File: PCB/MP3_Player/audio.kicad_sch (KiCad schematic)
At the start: 23 parts, among them J7 AudioPlugTRRS, J8 AudioPlugTRRS, U6 PCM5102AQPWRQ1

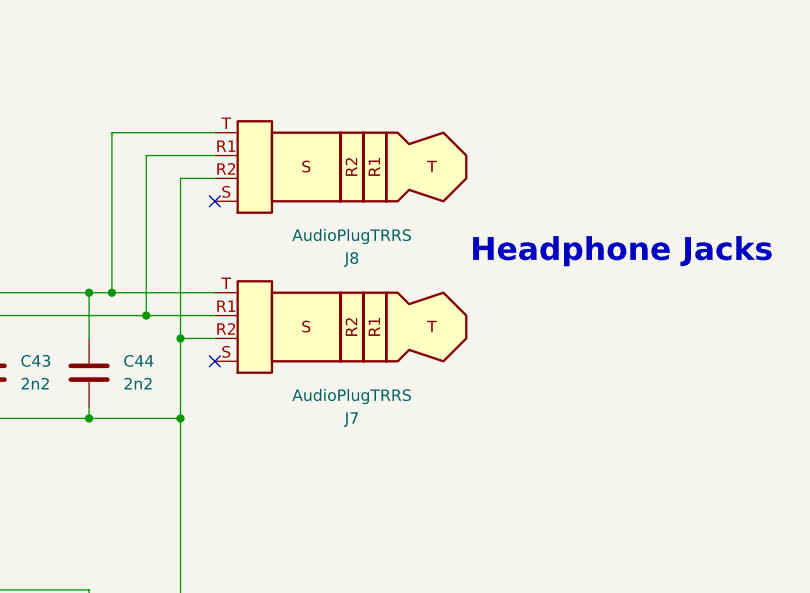
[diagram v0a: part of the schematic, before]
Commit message: PCB Routing
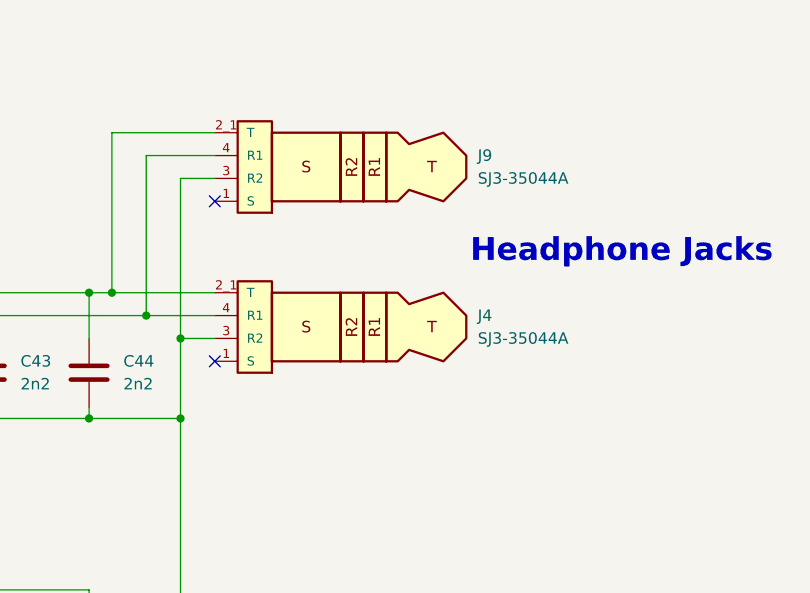
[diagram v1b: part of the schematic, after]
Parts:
- removed J7, J8: AudioPlugTRRS, SJ3-35044A:SAMESKY_SJ3-35044A, symbol Connector_Audio:AudioPlug4
- added J4, J9: SJ3-35044A, SJ3-35044A:SAMESKY_SJ3-35044A, symbol SJ3-35044A:SJ3-35044A
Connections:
- net GND: now also J4.3 (R2), J9.3 (R2)
- net LOUT: now also J4.2_1 (T), J4.2_2, J9.2_1 (T), J9.2_2
- net ROUT: now also J4.4 (R1), J9.4 (R1)

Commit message: PCB Routing
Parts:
- J4, J9: Mfr. Part # (none) -> SJ3-35044A; Store URL - Digikey (none) -> https://www.digikey.pt/pt/products/detail/same-sky-formerly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
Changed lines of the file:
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@@
 			)
 		)
-		(property "Datasheet" ""
+		(property "Datasheet" "https://www.sameskydevices.com/product/resource/sj3-35044a.pdf"
 			(at 229.87 71.12 0)
 			(hide yes)
@@
 				)
 				(justify bottom)
+			)
+		)
+		(property "Mfr. Part #" "SJ3-35044A"
+			(at 229.87 71.12 0)
+			(hide yes)
+			(show_name no)
+			(do_not_autoplace no)
+			(effects
+				(font
+					(size 1.27 1.27)
+				)
+			)
+		)
+		(property "Store URL - Digikey" "https://www.digikey.pt/pt/products/detail/same-sky-formerly-cui-devices/SJ3-35044A/24627965?s=N4IgTCBcDaIMoCkDMBaJBWADAFmwQRAF0BfIA"
+			(at 229.87 71.12 0)
+			(hide yes)
+			(show_name no)
+			(do_not_autoplace no)
+			(effects
+				(font
+					(size 1.27 1.27)
+				)
 			)
 		)
@@
 			)
 		)
-		(property "Datasheet" ""
+		(property "Datasheet" "https://www.sameskydevices.com/product/resource/sj3-35044a.pdf"
 			(at 229.87 53.34 0)
 			(hide yes)
@@
 			)
 		)
+		(property "Mfr. Part #" "SJ3-35044A"
+			(at 229.87 53.34 0)
+			(hide yes)
+			(show_name no)
+			(do_not_autoplace no)
+			(effects
+				(font
+					(size 1.27 1.27)
+				)
+			)
+		)
+		(property "Store URL - Digikey" "https://www.digikey.pt/pt/products/detail/same-sky-formerly-cui-devices/SJ3-35044A/24627965?s=N4IgTCBcDaIMoCkDMBaJBWADAFmwQRAF0BfIA"
+			(at 229.87 53.34 0)
+			(hide yes)
+			(show_name no)
+			(do_not_autoplace no)
+			(effects
+				(font
+					(size 1.27 1.27)
+				)
+			)
+		)
